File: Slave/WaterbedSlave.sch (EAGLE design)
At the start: 8 parts

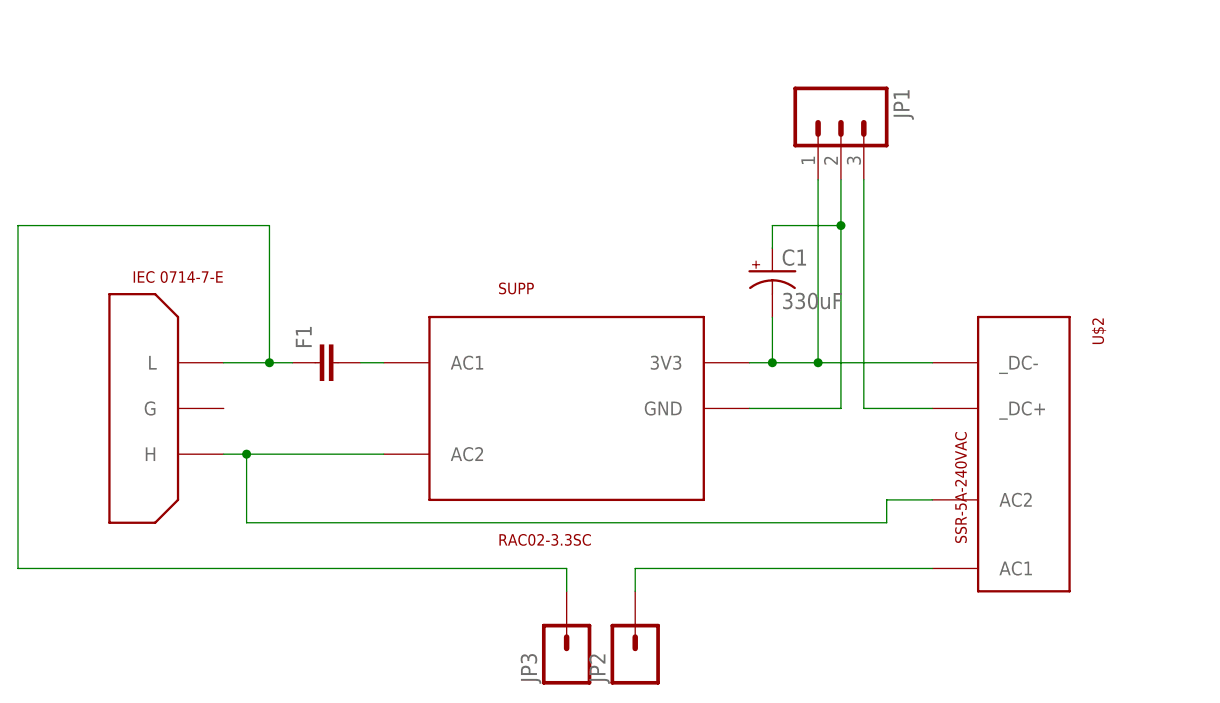
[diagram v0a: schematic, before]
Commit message: Update WaterbedSlave.sch
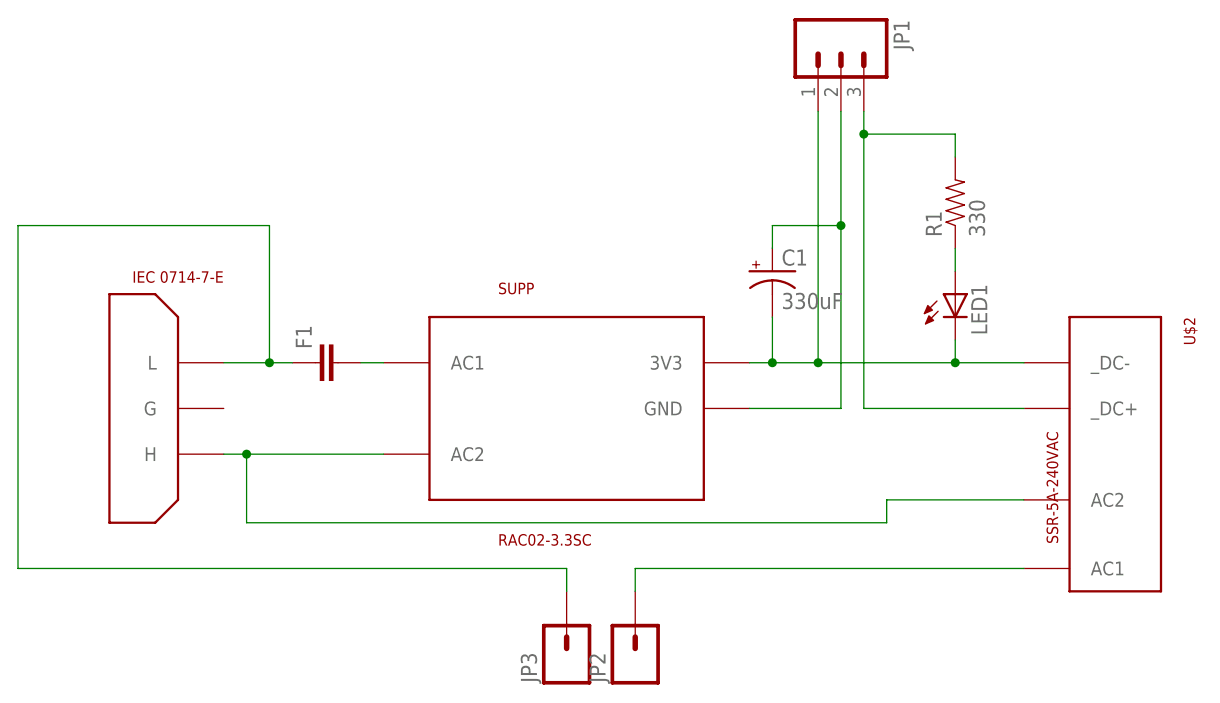
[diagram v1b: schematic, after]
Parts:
- added LED1: (no value), led:LEDCHIPLED_0805
- added R1: 330, SparkFun-Resistors:RESISTOR0805-RES
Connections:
- new net N$10: LED1.A, R1.1
- net GND: now also LED1.C
- net N$16: now also R1.2
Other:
- moved on the sheet: JP1, U$2
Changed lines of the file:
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@@
 <part name="JP2" library="SparkFun-Connectors" deviceset="M01" device="PTH_2MM"/>
 <part name="F1" library="SparkFun-Capacitors" deviceset="CAP" device="PTH1"/>
+<part name="LED1" library="led" deviceset="LED" device="CHIPLED_0805"/>
+<part name="R1" library="SparkFun-Resistors" deviceset="RESISTOR" device="0805-RES" value="330"/>
 </parts>
 <sheets>
@@
 </plain>
 <instances>
-<instance part="U$2" gate="G$1" x="111.76" y="55.88" rot="R270"/>
-<instance part="JP1" gate="G$1" x="91.44" y="93.98" rot="R270"/>
+<instance part="U$2" gate="G$1" x="121.92" y="55.88" rot="R270"/>
+<instance part="JP1" gate="G$1" x="91.44" y="101.6" rot="R270"/>
 <instance part="C1" gate="G$1" x="83.82" y="76.2"/>
 <instance part="U$3" gate="G$1" x="17.78" y="55.88" rot="MR180"/>
@@
 <instance part="JP2" gate="G$1" x="68.58" y="33.02" rot="R90"/>
 <instance part="F1" gate="G$1" x="35.56" y="66.04" rot="R90"/>
+<instance part="LED1" gate="G$1" x="104.14" y="73.66"/>
+<instance part="R1" gate="G$1" x="104.14" y="83.82" rot="R90"/>
 </instances>
 <busses>
@@
 <pinref part="JP1" gate="G$1" pin="1"/>
 <pinref part="U$2" gate="G$1" pin="_DC-"/>
-<wire x1="88.9" y1="66.04" x2="88.9" y2="86.36" width="0.1524" layer="91"/>
-<wire x1="101.6" y1="66.04" x2="88.9" y2="66.04" width="0.1524" layer="91"/>
+<wire x1="88.9" y1="66.04" x2="88.9" y2="93.98" width="0.1524" layer="91"/>
+<wire x1="111.76" y1="66.04" x2="104.14" y2="66.04" width="0.1524" layer="91"/>
 <junction x="88.9" y="66.04"/>
 <pinref part="C1" gate="G$1" pin="-"/>
+<wire x1="104.14" y1="66.04" x2="88.9" y2="66.04" width="0.1524" layer="91"/>
 <wire x1="83.82" y1="66.04" x2="83.82" y2="71.12" width="0.1524" layer="91"/>
 <wire x1="81.28" y1="66.04" x2="83.82" y2="66.04" width="0.1524" layer="91"/>
@@
 <junction x="83.82" y="66.04"/>
 <pinref part="SUPP" gate="G$1" pin="3V3"/>
+<pinref part="LED1" gate="G$1" pin="C"/>
+<wire x1="104.14" y1="68.58" x2="104.14" y2="66.04" width="0.1524" layer="91"/>
+<junction x="104.14" y="66.04"/>
 </segment>
 </net>
@@
 <pinref part="SUPP" gate="G$1" pin="GND"/>
 <pinref part="C1" gate="G$1" pin="+"/>
-<wire x1="91.44" y1="81.28" x2="91.44" y2="86.36" width="0.1524" layer="91"/>
+<wire x1="91.44" y1="81.28" x2="91.44" y2="93.98" width="0.1524" layer="91"/>
 <wire x1="83.82" y1="78.74" x2="83.82" y2="81.28" width="0.1524" layer="91"/>
 <wire x1="83.82" y1="81.28" x2="91.44" y2="81.28" width="0.1524" layer="91"/>
@@
 <segment>
 <pinref part="JP1" gate="G$1" pin="3"/>
-<wire x1="93.98" y1="86.36" x2="93.98" y2="60.96" width="0.1524" layer="91"/>
+<wire x1="93.98" y1="93.98" x2="93.98" y2="91.44" width="0.1524" layer="91"/>
 <pinref part="U$2" gate="G$1" pin="_DC+"/>
-<wire x1="93.98" y1="60.96" x2="101.6" y2="60.96" width="0.1524" layer="91"/>
+<wire x1="93.98" y1="91.44" x2="93.98" y2="60.96" width="0.1524" layer="91"/>
+<wire x1="93.98" y1="60.96" x2="111.76" y2="60.96" width="0.1524" layer="91"/>
+<pinref part="R1" gate="G$1" pin="2"/>
+<wire x1="104.14" y1="88.9" x2="104.14" y2="91.44" width="0.1524" layer="91"/>
+<wire x1="104.14" y1="91.44" x2="93.98" y2="91.44" width="0.1524" layer="91"/>
+<junction x="93.98" y="91.44"/>
 </segment>
 </net>
@@
 <wire x1="96.52" y1="48.26" x2="96.52" y2="50.8" width="0.1524" layer="91"/>
 <pinref part="U$2" gate="G$1" pin="AC2"/>
-<wire x1="96.52" y1="50.8" x2="101.6" y2="50.8" width="0.1524" layer="91"/>
+<wire x1="96.52" y1="50.8" x2="111.76" y2="50.8" width="0.1524" layer="91"/>
 <pinref part="U$3" gate="G$1" pin="H"/>
 <wire x1="22.86" y1="55.88" x2="25.4" y2="55.88" width="0.1524" layer="91"/>
@@
 <segment>
 <pinref part="U$2" gate="G$1" pin="AC1"/>
-<wire x1="101.6" y1="43.18" x2="68.58" y2="43.18" width="0.1524" layer="91"/>
+<wire x1="111.76" y1="43.18" x2="68.58" y2="43.18" width="0.1524" layer="91"/>
 <wire x1="68.58" y1="43.18" x2="68.58" y2="40.64" width="0.1524" layer="91"/>
 <pinref part="JP2" gate="G$1" pin="1"/>
@@
 </segment>
 </net>
+<net name="N$10" class="0">
+<segment>
+<pinref part="R1" gate="G$1" pin="1"/>
+<pinref part="LED1" gate="G$1" pin="A"/>
+<wire x1="104.14" y1="78.74" x2="104.14" y2="76.2" width="0.1524" layer="91"/>
+</segment>
+</net>
